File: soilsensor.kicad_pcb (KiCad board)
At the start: 2 copper layers, 29 parts, among them J1 CONN_01X06, J2 BATT_CONN, P1 USB_OTG, U1 DS18B20, U2 RFD77101, U3 BQ24075, U4 MCP1700-3002E_SOT23, U5 TLC555

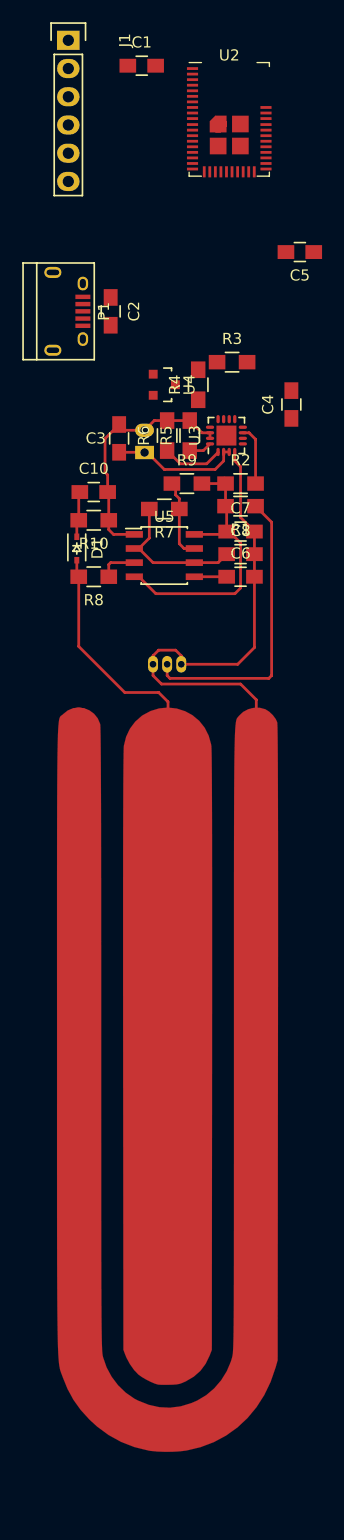
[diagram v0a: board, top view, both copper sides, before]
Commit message: finish pcb
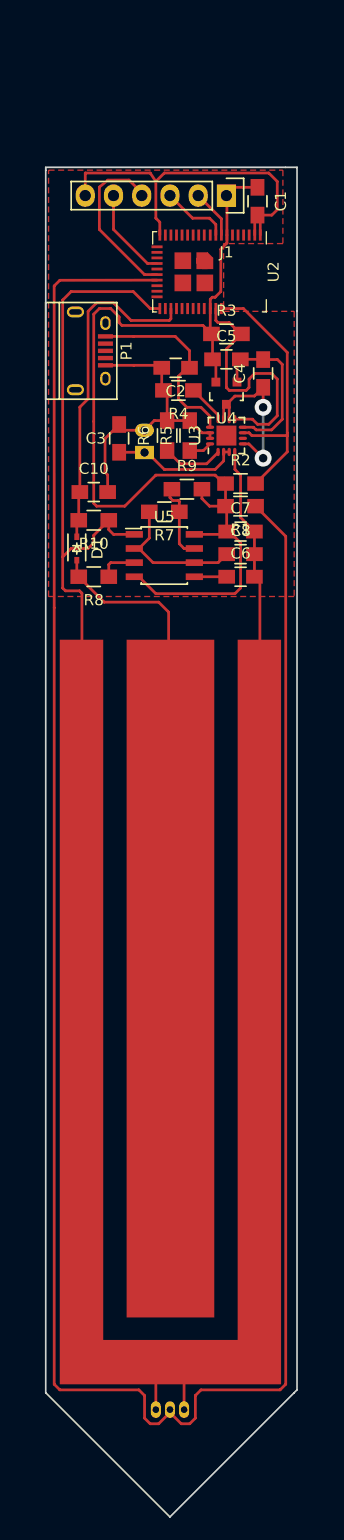
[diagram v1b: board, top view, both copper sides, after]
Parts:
- moved U1 67.1 mm to (103.4, 144.3)
- moved J1 19.9 mm to (109.7, 35.1), turned to 180 degrees
- moved C1 16.0 mm to (112.5, 35.6), turned to 270 degrees
- moved U2 13.8 mm to (108.2, 41.9), turned to 270 degrees
- moved C5 11.7 mm to (109.7, 49.8), turned to 0 degrees
- moved C2 7.74 mm to (105.2, 50.5), turned to 180 degrees
- moved C9 6.10 mm to (104.6, 108.5)
- moved U4 5.64 mm to (109.7, 52.8), turned to 180 degrees
- moved P1 4.10 mm to (97.3, 49.0)
- moved C4 3.78 mm to (113.0, 51.1)
- moved R3 2.59 mm to (109.7, 47.5)
- moved R4 1.85 mm to (105.4, 52.6), turned to 180 degrees
- moved R9 0.51 mm to (106.2, 61.5)
- moved R7 0.25 mm to (104.1, 63.5)
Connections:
- U2 pad 24: /CapacitiveSoilSensor/SensorOut -> Net-(U2-Pad24)
- U2 pad 30: Net-(U2-Pad30) -> GND
- U2 pad 32: Net-(U2-Pad32) -> /CapacitiveSoilSensor/SensorOut
- U2 pad 39: Net-(U2-Pad39) -> VDD
- U2 pad 42: Net-(U2-Pad42) -> GND
- U2 pad 43: Net-(U2-Pad43) -> GND
- U2 pad 44: Net-(U2-Pad44) -> GND
- U2 pad 45: Net-(U2-Pad45) -> GND
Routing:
- net GND: track 67.0 -> 295.4 mm
- net Net-(R1-Pad1): track 26.5 -> 215.6 mm
- net VDD: track 25.8 -> 90.3 mm
- net /CapacitiveSoilSensor/SensorOut: track 4.28 -> 30.3 mm
- net /PowerMgmt/~CHG: track 0.00 -> 22.9 mm
- net /PowerMgmt/~PGOOD: track 5.37 -> 24.6 mm
- net Net-(C2-Pad1): track 0.00 -> 17.5 mm
- net Net-(C4-Pad1): track 0.00 -> 15.5 mm, vias 0 -> 2
- net /GPIO0: track 0.00 -> 15.4 mm
- net /GPIO1: track 0.00 -> 8.23 mm
- net /SWDCLK: track 0.00 -> 6.15 mm
- net Net-(C9-Pad1): track 20.0 -> 15.4 mm
- net /SWDIO/RESET: track 0.00 -> 4.42 mm
- net Net-(R4-Pad1): track 0.00 -> 3.80 mm
- net Net-(R7-Pad1): track 7.35 -> 8.81 mm
- added copper zone on F.Cu, net GND
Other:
- board outline added: 22.6 x 121.4 mm
